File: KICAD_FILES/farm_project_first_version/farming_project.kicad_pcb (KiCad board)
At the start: 2 copper layers, 59.5 x 94 mm, 17 parts, among them J1 Arduino_MKRWAN_SHIELD, J10 Capteur_temperature_sous_sol, J2 Capteur de pression, J3 Capteur de luminosite, J4 Capteur_de_CO2, J5 Capteur_humidite_sous_sol_10cm, J6 Capteur_humidite_sous_sol_20cm, J7 Capteur_humidite_sous_sol_30cm, J8 DHT22, J9 battery_input

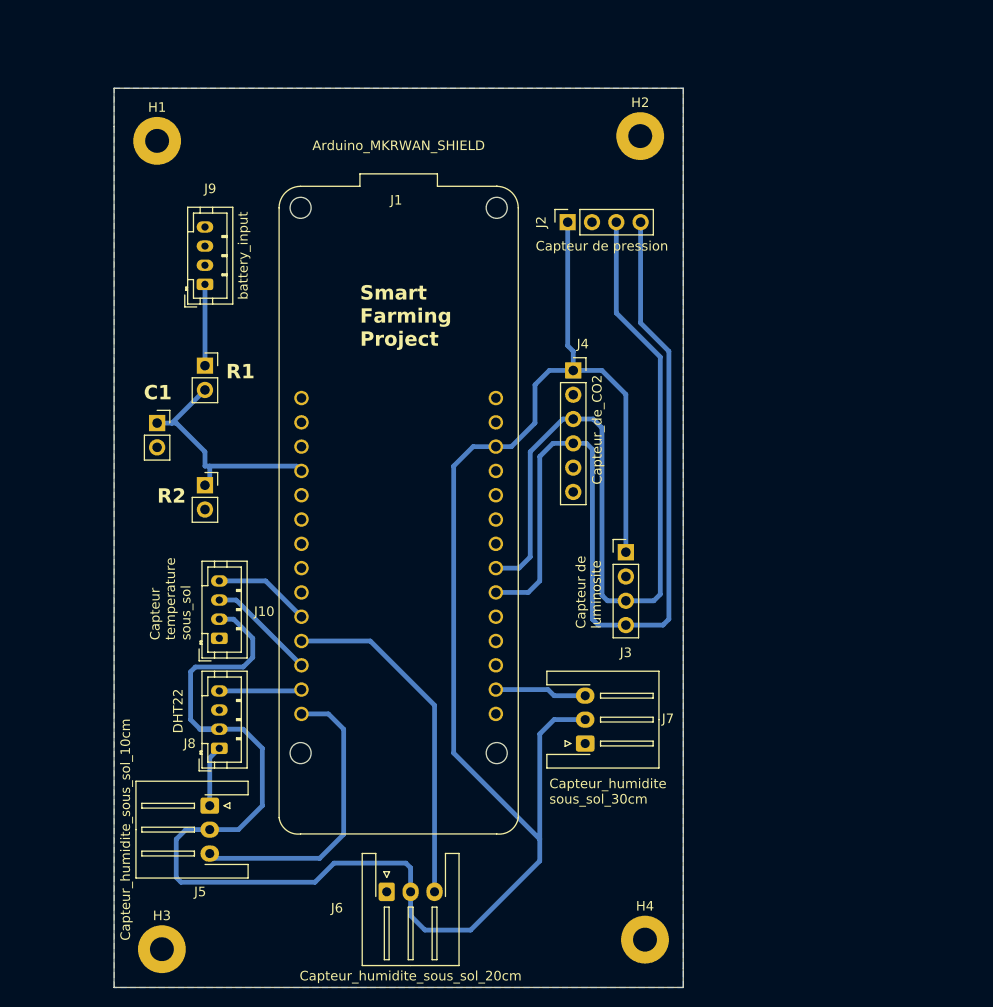
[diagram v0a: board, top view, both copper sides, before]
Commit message: deuxieme version PCB
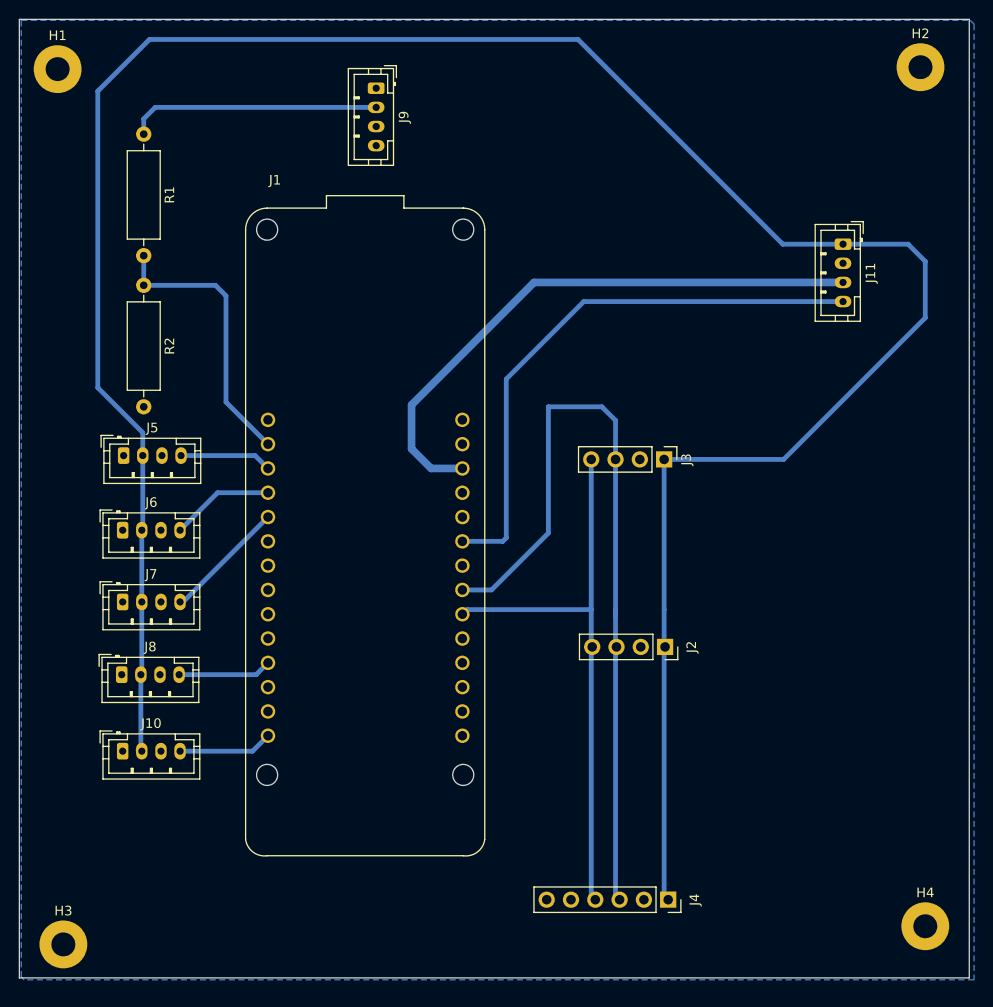
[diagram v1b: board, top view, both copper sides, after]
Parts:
- removed C1: 100n, Connector_PinSocket_2.54mm:PinSocket_1x02_P2.54mm_Vertical
- added J11: regulateur_tension, Connector_JST:JST_PH_B4B-PH-K_1x04_P2.00mm_Vertical, F.Cu at (186.7, 62.8)
- J5, J6, J7: footprint Connector_JST:JST_XH_S3B-XH-A-1_1x03_P2.50mm_Horizontal -> Connector_JST:JST_PH_B4B-PH-K_1x04_P2.00mm_Vertical
- R1, R2: footprint Connector_PinSocket_2.54mm:PinSocket_1x02_P2.54mm_Vertical -> Resistor_THT:R_Axial_DIN0309_L9.0mm_D3.2mm_P12.70mm_Horizontal
- moved J4 56.2 mm to (168.4, 131.3), turned to -90 degrees
- moved J7 50.6 mm to (111.4, 100.2), turned to 0 degrees
- moved J6 46.8 mm to (111.4, 92.7)
- moved J2 45.6 mm to (168.1, 104.9), turned to -90 degrees
- moved J5 37.7 mm to (111.5, 84.9), turned to 0 degrees
- moved H2 30.2 mm to (194.8, 44.3)
- moved H4 29.3 mm to (195.3, 134.1)
- moved J9 27.2 mm to (137.9, 46.5), turned to -90 degrees
- moved R1 25.0 mm to (113.6, 51.3), turned to -90 degrees
- moved R2 21.9 mm to (113.6, 67.1), turned to -90 degrees
- moved J10 15.5 mm to (111.4, 115.8), turned to 0 degrees
- moved H1 12.8 mm to (104.6, 44.5)
- moved J8 12.8 mm to (111.3, 107.8), turned to 0 degrees
- moved J3 10.5 mm to (168.0, 85.3), turned to -90 degrees
- moved H3 10.3 mm to (105.2, 136.0)
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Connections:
- J1 pad 2: /DAC0/A0 -> /A0
- J1 pad 23: /TX -> /D14
- J10 pad 2: VCC -> VOUT
- J10 pad 3: /D3 -> unconnected-(J10-Pin_3-Pad3)
- J10 pad 4: /D1 -> /D5
- J2 pad 1: VCC -> VOUT
- J3 pad 1: VCC -> VOUT
- J4 pad 1: VCC -> VOUT
- J5 pad 2: VCC -> VOUT
- J5 pad 3: /D5 -> unconnected-(J5-Pin_3-Pad3)
- J6 pad 2: VCC -> VOUT
- J6 pad 3: /D2 -> unconnected-(J6-Pin_3-Pad3)
- J7 pad 2: VCC -> VOUT
- J7 pad 3: /D7 -> unconnected-(J7-Pin_3-Pad3)
- J8 pad 2: VCC -> VOUT
- J8 pad 4: /D4 -> /D2
- J9 pad 1: Vbat -> GND
- J9 pad 2: GND -> Vbat
- R1 pad 2: /A2 -> /A0
- R2 pad 1: /A2 -> /A0
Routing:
- net VOUT: track 0.00 -> 255.4 mm
- net VCC: track 214.9 -> 61.2 mm
- net /D14: track 0.00 -> 59.9 mm
- net /SDA: track 93.4 -> 59.9 mm
- net /A0: track 0.00 -> 29.5 mm
- net /D2: track 36.2 -> 9.80 mm
- net /D5: track 31.3 -> 9.86 mm
- net Vbat: track 8.50 -> 26.4 mm
- net /A2: track 25.1 -> 10.8 mm
- net /A3: track 0.00 -> 12.9 mm
- net /D3: track 11.4 -> 0.00 mm
- net /D1: track 10.1 -> 0.00 mm
- net /D7: track 9.73 -> 0.00 mm
- net /A1: track 0.00 -> 9.65 mm
- net /D4: track 8.65 -> 0.00 mm
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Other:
- board size 59.5 x 94 mm -> 99.3 x 100.2 mm
- board text removed: "C1"
- board text removed: "Capteur de luminosite"
- board text removed: "Capteur temperature sous_sol"
- board text removed: "Capteur_humidite sous_sol_30cm"
- board text removed: "R1"
- board text removed: "R2"
- board text removed: "Smart Farming Project"
